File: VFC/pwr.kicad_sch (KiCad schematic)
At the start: 44 parts, among them J2 USB4940-00-A_REVA, U10 USBLC6-2SC6, U3 AP2112K-3.3TRG1

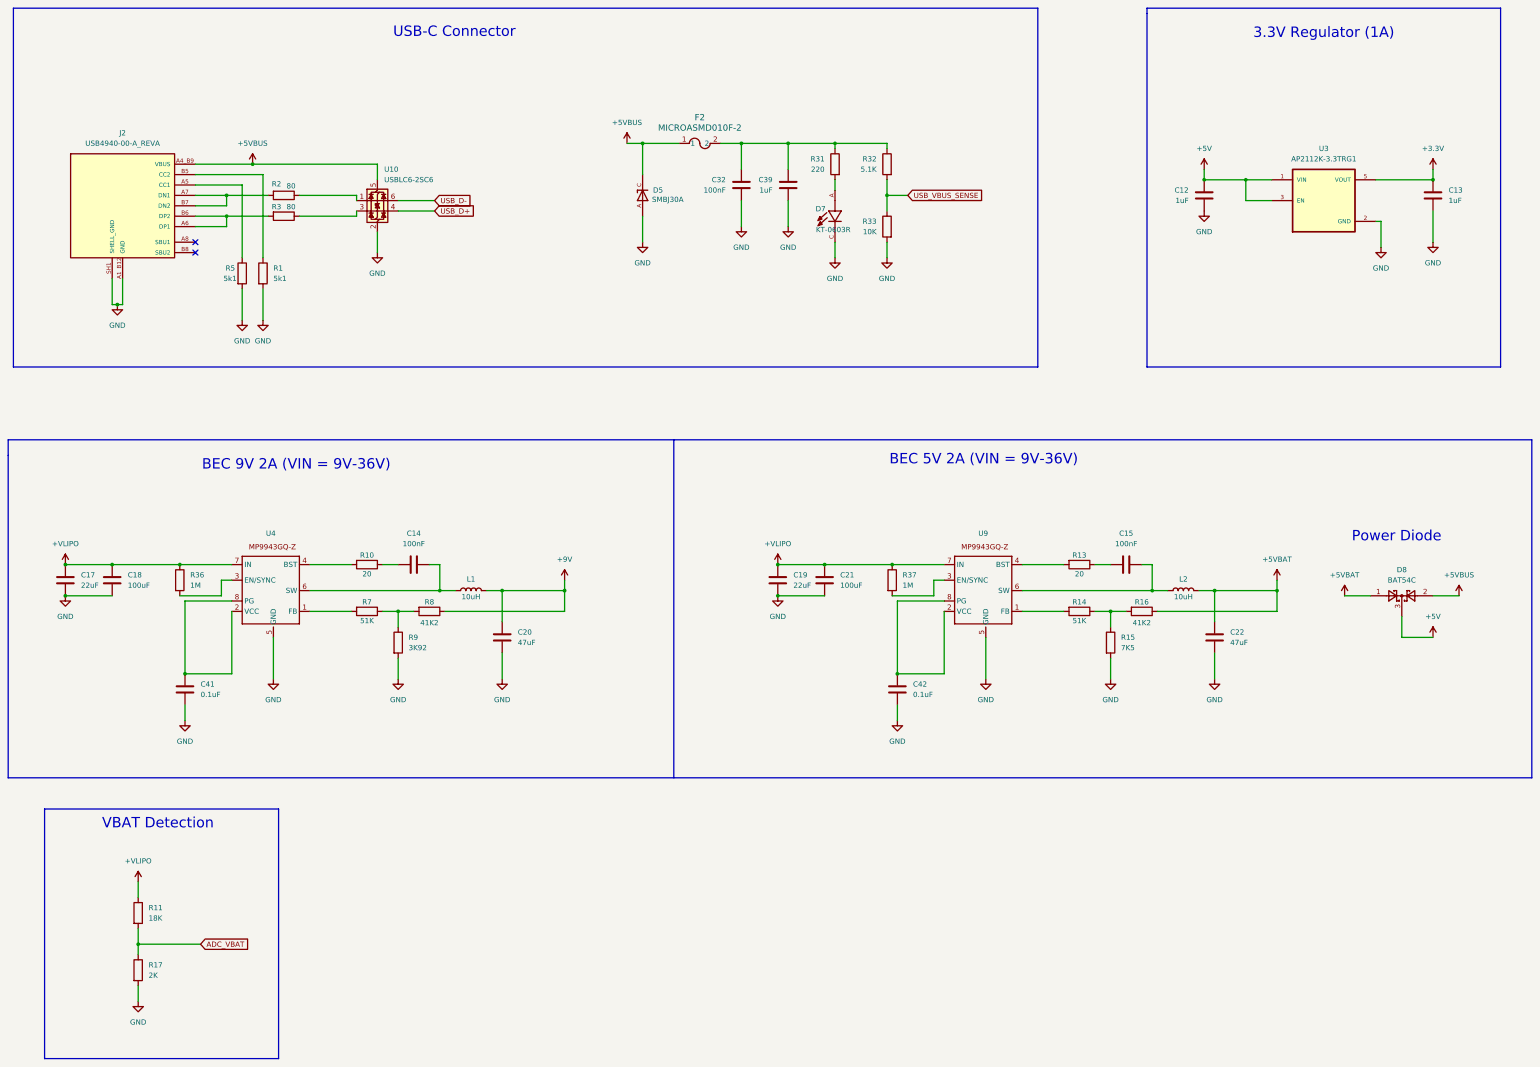
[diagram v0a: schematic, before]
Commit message: VFC PCB traces update
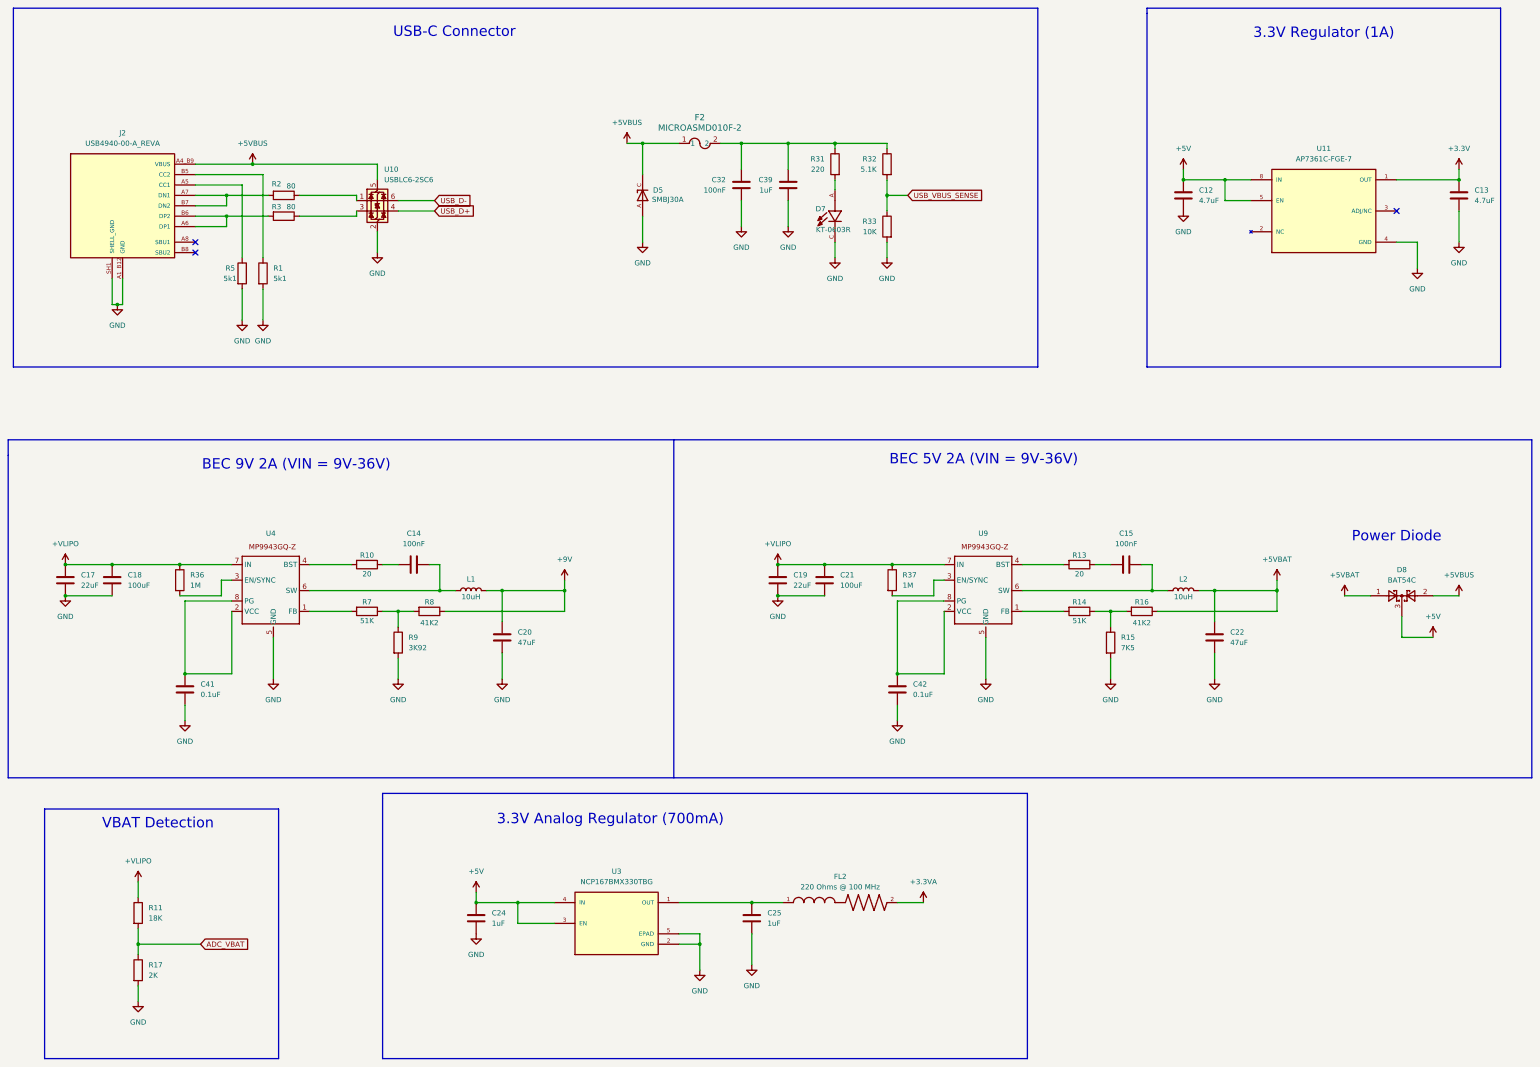
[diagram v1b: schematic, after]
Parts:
- removed U3: AP2112K-3.3TRG1, AP2112K-3.3TRG1:SOT95P285X140-5N, symbol AP2112K-3.3TRG1:AP2112K-3.3TRG1
- added C24, C25: 1uF, Capacitor_SMD:C_0402_1005Metric, symbol Device:C
- added FL2: 220 Ohms @ 100 MHz, BLM18PG221SN1D:BEADC1608X95N, symbol BLM18PG221SN1D:BLM18PG221SN1D
- added U11: AP7361C-FGE-7, AP7361C-FGE-7:SON65P300X300X63-9N, symbol AP7361C-FGE-7:AP7361C-FGE-7
- added U3: NCP167BMX330TBG, NCP167BMX330TBG:VREG_NCP167BMX330TBG, symbol NCP167BMX330TBG:NCP167BMX330TBG
- C12, C13: value 1uF -> 4.7uF
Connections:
- net +3.3V: now also U11.1 (OUT)
- net +5V: now also C24.1, U11.5 (EN), U11.8 (IN), U3.3 (EN), U3.4 (IN)
- net GND: now also C24.2, C25.2, U11.4 (GND), U11.9 (GND), U3.2 (GND), U3.5 (EPAD)
- new net: C25.1, FL2.1, U3.1 (OUT)
- new net: U11.2 (NC), U11.6 (NC), U11.7 (NC)
- new net +3.3VA: FL2.2
- no-connect marks 2 -> 3
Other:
- note added: "3.3V Analog Regulator (700mA)"
- moved on the sheet: C12, C13
